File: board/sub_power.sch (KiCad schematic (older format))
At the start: 1 part, among them U201 XC3S200-TQ144

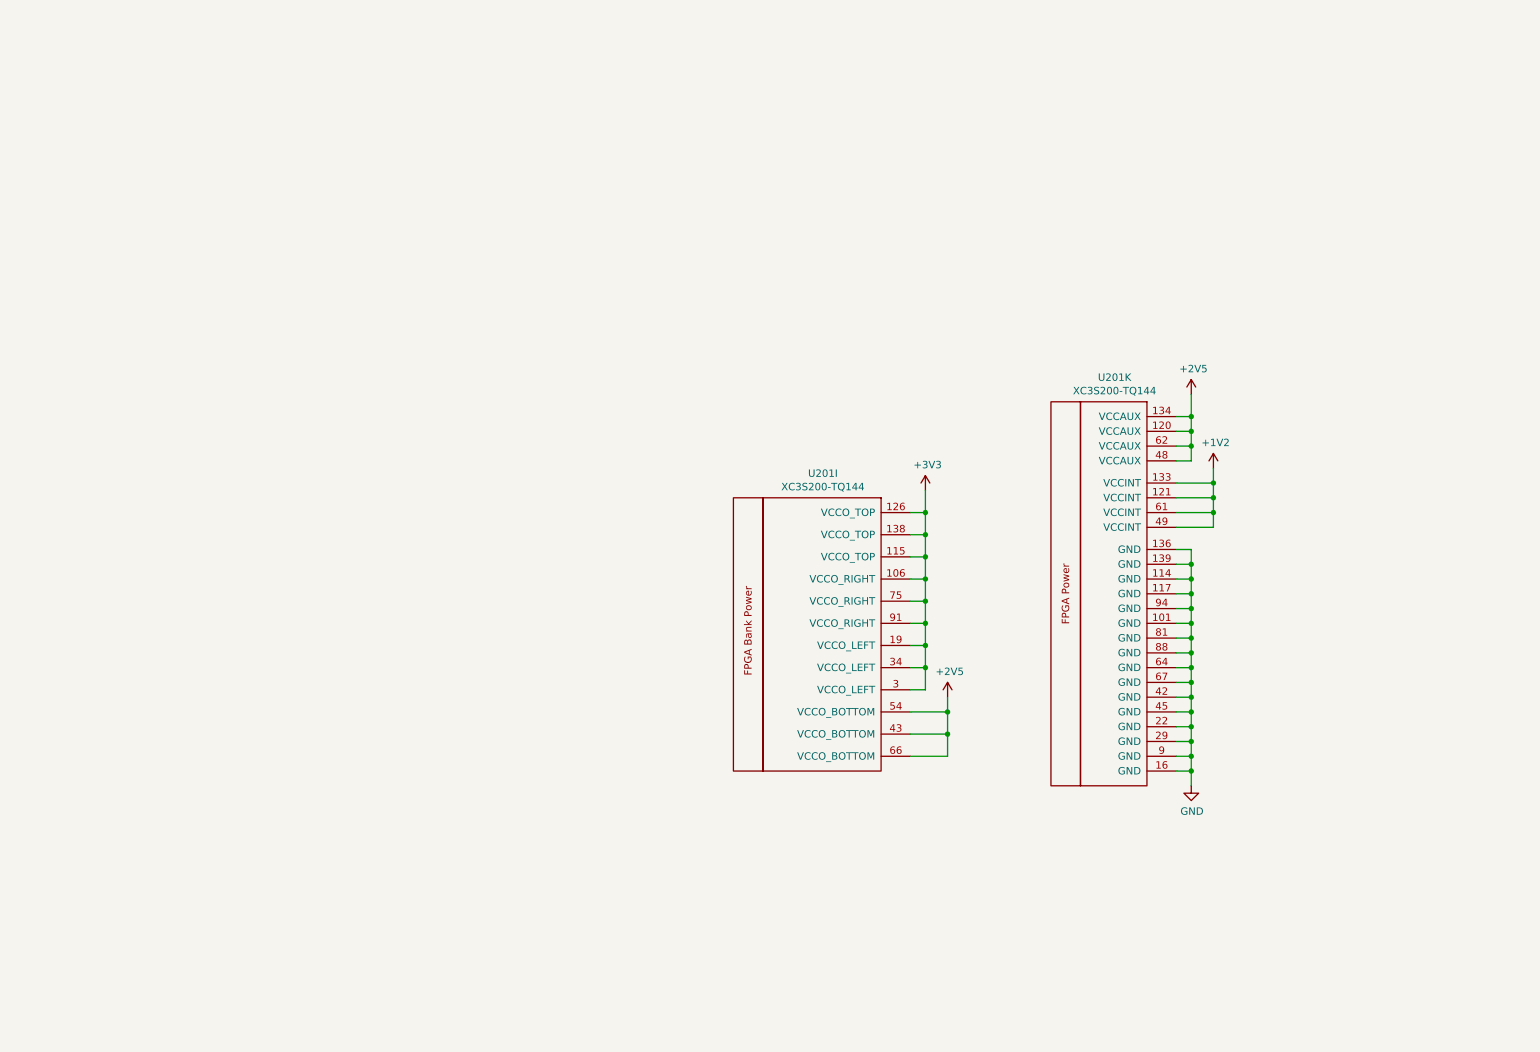
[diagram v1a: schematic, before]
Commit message: Schematics mostly complete
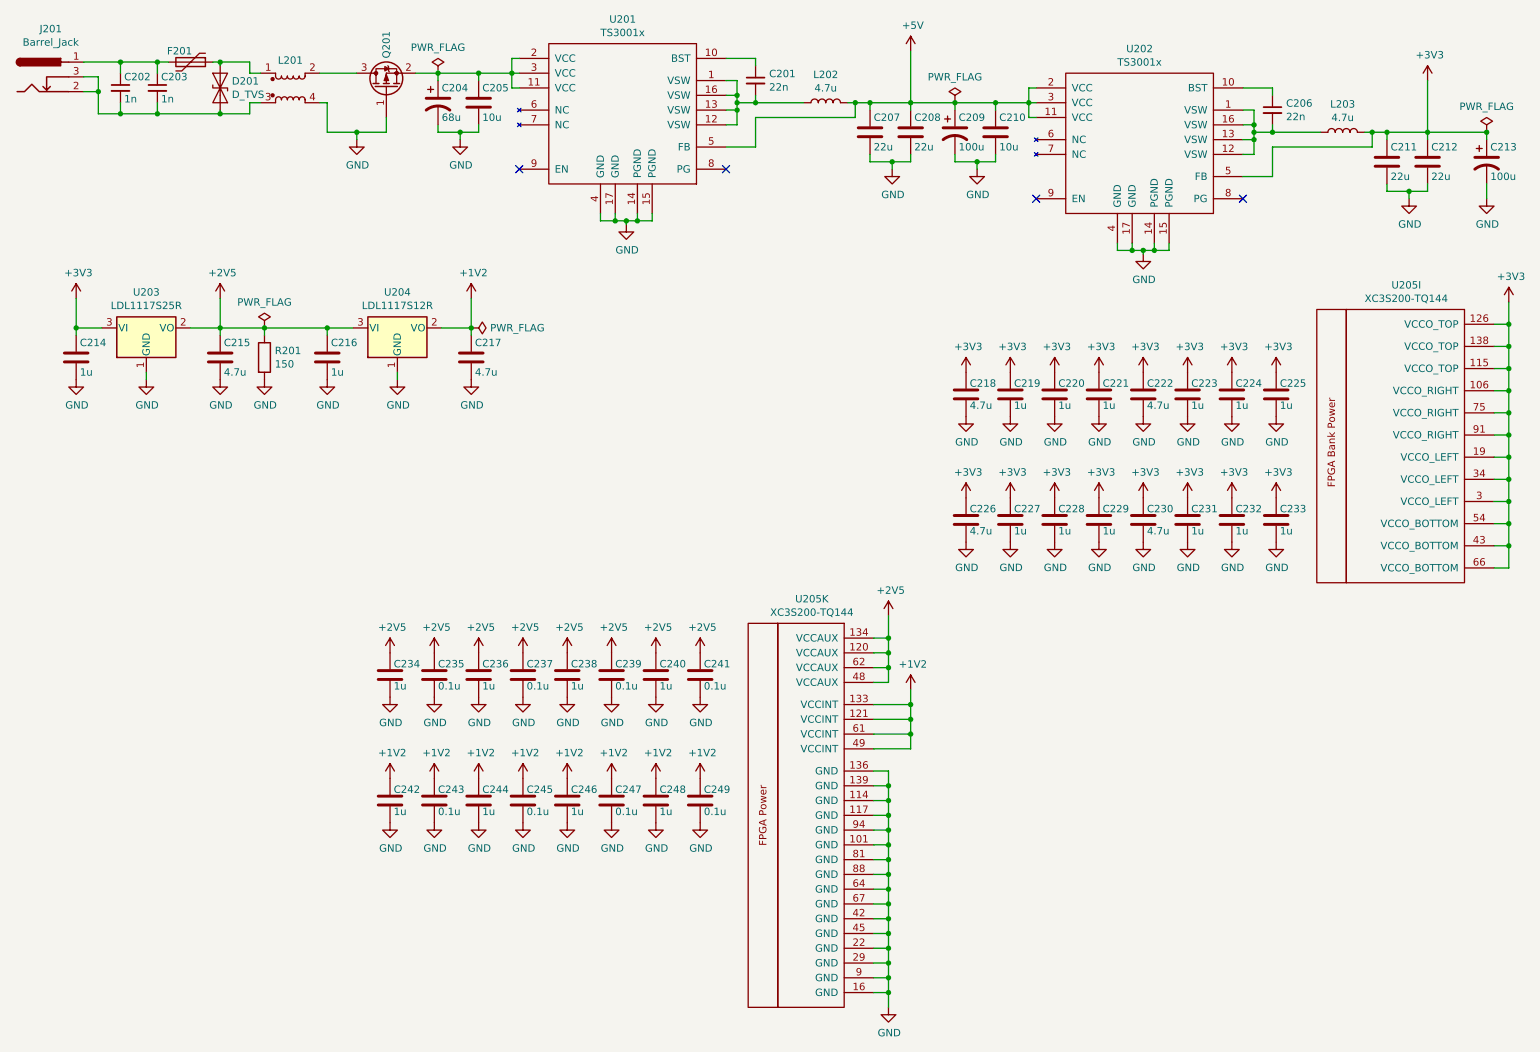
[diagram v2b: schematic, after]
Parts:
- added C201, C206: 22n, symbol Device:C_Small
- added C202, C203: 1n, symbol Device:C_Small
- added C204: 68u, symbol Device:CP1
- added C205, C210: 10u, symbol Device:C
- added C207, C208, C211, C212: 22u, symbol Device:C
- added C209, C213: 100u, symbol Device:CP1
- added C214, C216, C219, C220, C221, C223, C224, C225, C227, C228, C229, C231, C232, C233, C234, C236, C238, C240, C242, C244, C246, C248: 1u, symbol Device:C
- added C215, C217, C218, C222, C226, C230: 4.7u, symbol Device:C
- added C235, C237, C239, C241, C243, C245, C247, C249: 0.1u, symbol Device:C
- added D201: D_TVS, symbol Device:D_TVS
- added F201: Polyfuse, symbol Device:Polyfuse
- added J201: Barrel_Jack, symbol Connector_Specialized:Barrel_Jack
- added L201: L_Coupled, symbol Device:L_Coupled
- added L202, L203: 4.7u, symbol Device:L
- added Q201: Q_PMOS_GSD, symbol Device:Q_PMOS_GSD
- added R201: 150, symbol Device:R
- added U201, U202: TS3001x, symbol quokka:TS3001x
- added U203: LDL1117S25R, symbol Regulator_Linear:TLV1117-33
- added U204: LDL1117S12R, symbol Regulator_Linear:TLV1117-33
- renumbered U201 to U205
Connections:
- net +1V2: now also C217.1, C242.1, C243.1, C244.1, C245.1, C246.1, C247.1, C248.1, C249.1, U204.2 (VO)
- net +2V5: now also C215.1, C216.1, C234.1, C235.1, C236.1, C237.1, C238.1, C239.1, C240.1, C241.1, R201.1, U203.2 (VO), U204.3 (VI); no longer U205.43 (VCCO_BOTTOM), U205.54 (VCCO_BOTTOM), U205.66 (VCCO_BOTTOM)
- net +3V3: now also U205.43 (VCCO_BOTTOM), U205.54 (VCCO_BOTTOM), U205.66 (VCCO_BOTTOM), C211.1, C212.1, C213.1, C214.1, C218.1, C219.1, C220.1, C221.1, C222.1, C223.1, C224.1, C225.1, C226.1, C227.1, C228.1, C229.1, C230.1, C231.1, C232.1, C233.1, L203.2, U202.5 (FB), U203.3 (VI)
- net GND: now also C204.2, C205.2, C207.2, C208.2, C209.2, C210.2, C211.2, C212.2, C213.2, C214.2, C215.2, C216.2, C217.2, C218.2, C219.2, C220.2, C221.2, C222.2, C223.2, C224.2, C225.2, C226.2, C227.2, C228.2, C229.2, C230.2, C231.2, C232.2, C233.2, C234.2, C235.2, C236.2, C237.2, C238.2, C239.2, C240.2, C241.2, C242.2, C243.2, C244.2, C245.2, C246.2, C247.2, C248.2, C249.2, L201.4, Q201.1 (G), R201.2, U201.14 (PGND), U201.15 (PGND), U201.17 (GND), U201.4 (GND), U202.14 (PGND), U202.15 (PGND), U202.17 (GND), U202.4 (GND), U203.1 (GND), U204.1 (GND)
- new net: C201.2, L202.1, U201.1 (VSW), U201.12 (VSW), U201.13 (VSW), U201.16 (VSW)
- new net: C201.1, U201.10 (BST)
- new net: C204.1, C205.1, Q201.2 (S), U201.11 (VCC), U201.2 (VCC), U201.3 (VCC)
- new net: L201.2, Q201.3 (D)
- new net: C202.1, C203.1, F201.2, J201.1
- new net: C202.2, C203.2, D201.2 (A2), J201.2, J201.3, L201.3
- new net: D201.1 (A1), F201.1, L201.1
- new net: C206.2, L203.1, U202.1 (VSW), U202.12 (VSW), U202.13 (VSW), U202.16 (VSW)
- new net: C206.1, U202.10 (BST)
- new net +5V: C207.1, C208.1, C209.1, C210.1, L202.2, U201.5 (FB), U202.11 (VCC), U202.2 (VCC), U202.3 (VCC)
- no-connect marks 0 -> 4
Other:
- moved on the sheet: U205I, U205K
